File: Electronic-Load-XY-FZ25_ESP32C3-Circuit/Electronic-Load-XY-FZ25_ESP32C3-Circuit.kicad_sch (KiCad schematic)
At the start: 15 parts, among them IC1 BD5334G-TR, J1 Banana-Socket, J2 Banana-Socket, J3 Banana-Socket, J4 Banana-Socket, J5 Conn_1x2_PH, J6 Conn_1x4_PH, J7 Conn_1x2_PH, J8 Conn_1x3_PH, J9 Conn_1x2_PH, Q1 AO3415, U2 Adafruit INA228, U3 SEEEDUINO-XIAO-ESP32C3

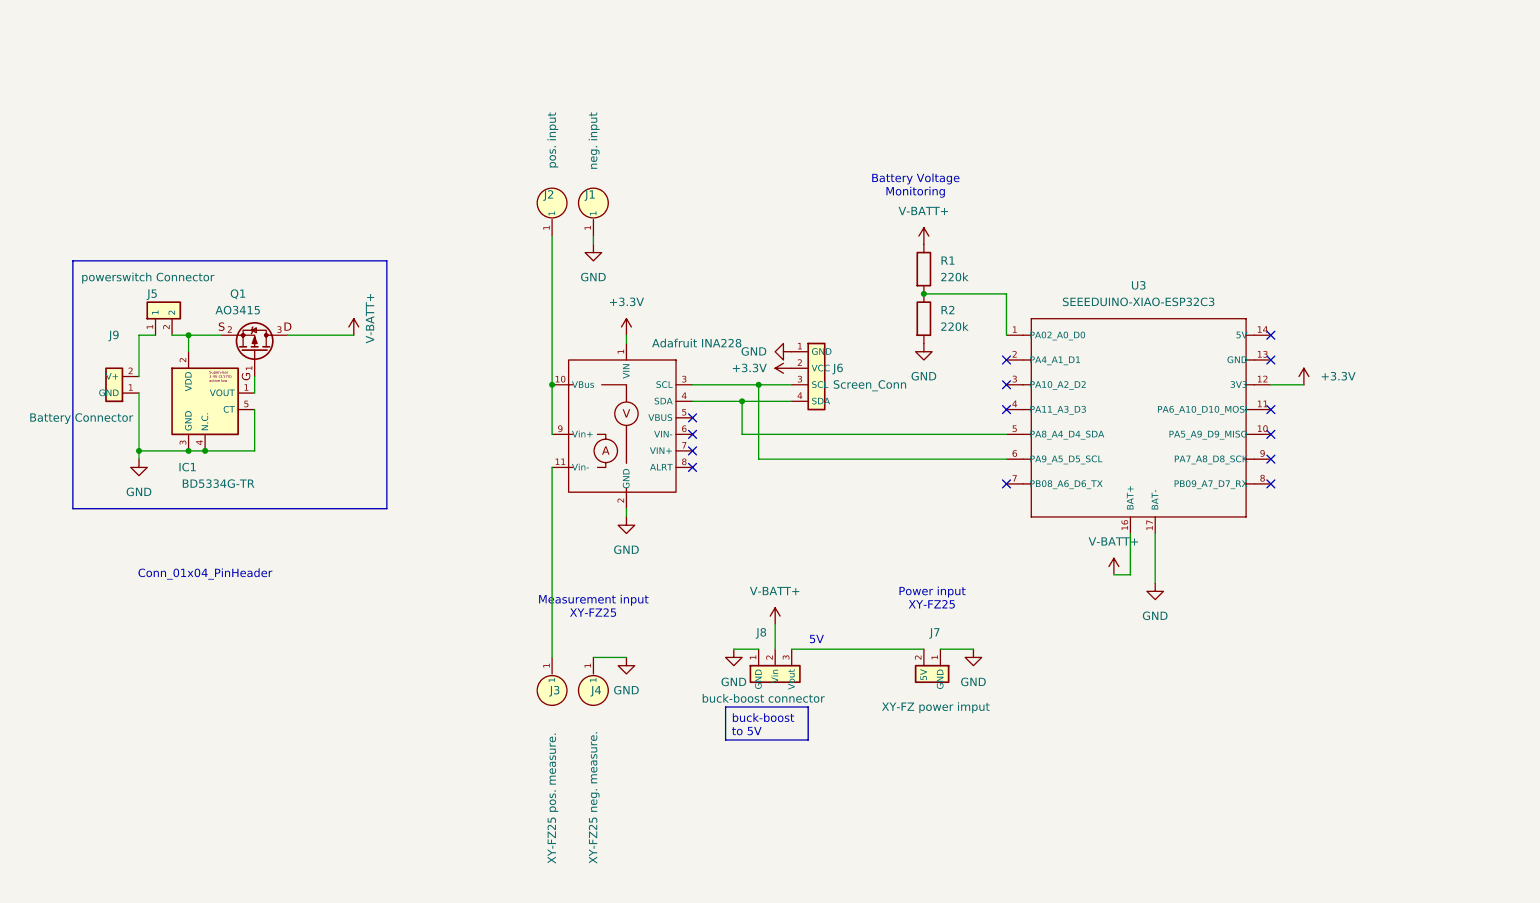
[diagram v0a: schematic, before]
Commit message: Add faulty first design
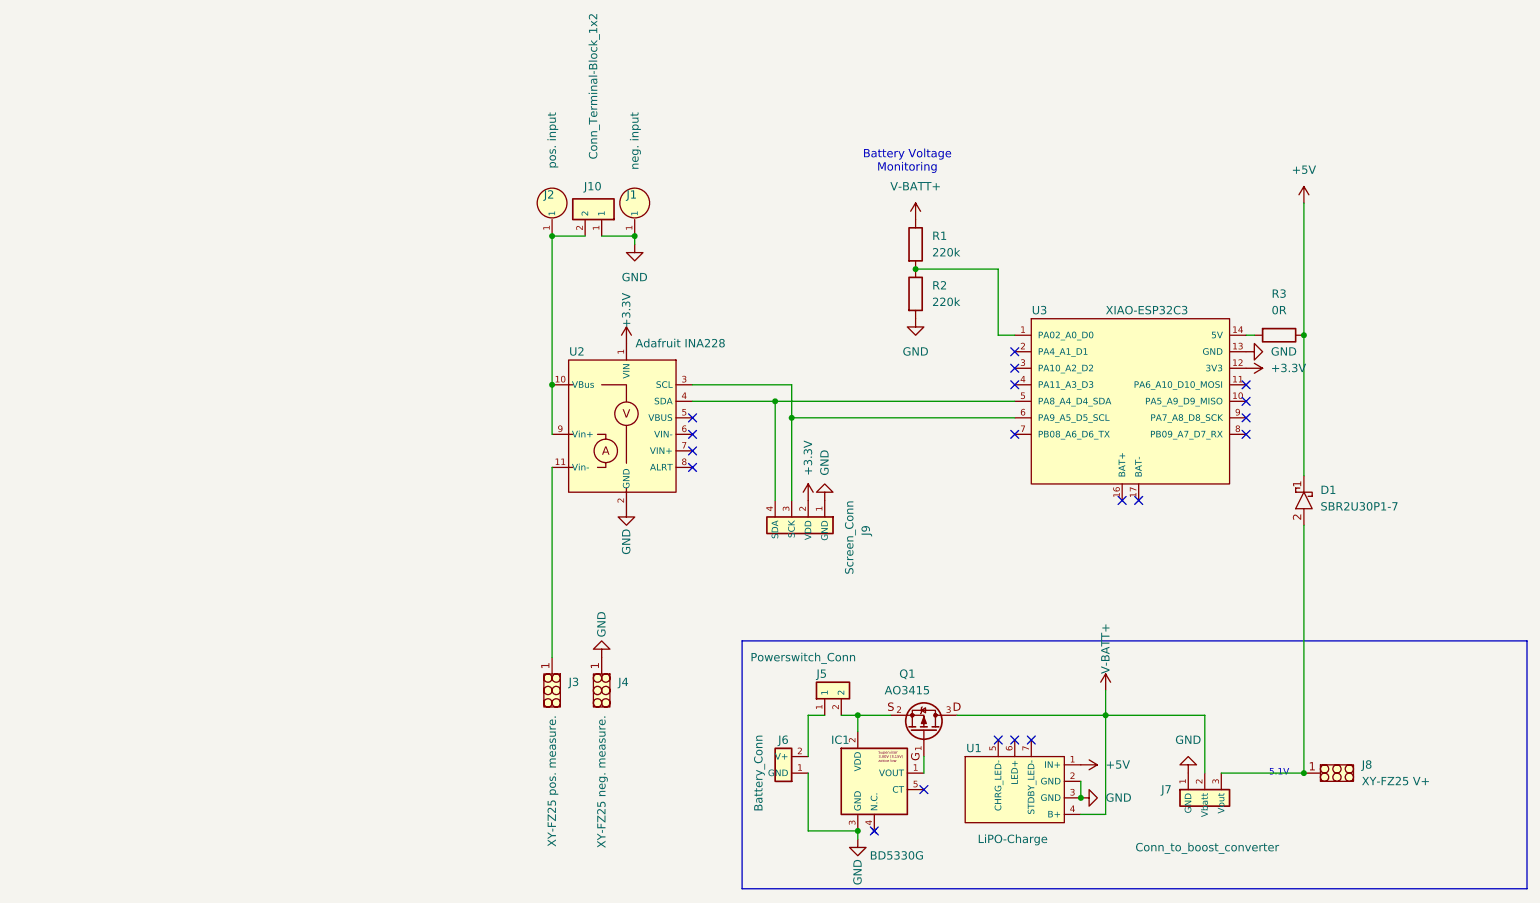
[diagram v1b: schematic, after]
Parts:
- removed IC1: BD5334G-TR, Marcus-PCB-Library:SOT95P280X125-5N, symbol Marcus-PCB-Library:BD5334G-TR
- removed J3, J4: Banana-Socket, Marcus-PCB-Library:banana-socket, symbol Marcus-PCB-Library:Banana-Socket
- removed J7: Conn_1x2_PH, Marcus-PCB-Library:Conn_1x2_PH, symbol Marcus-PCB-Library:Conn_1x2_PH
- removed J8: Conn_1x3_PH, Marcus-PCB-Library:Conn_1x3_PH, symbol Marcus-PCB-Library:Conn_1x3_PH
- added D1: SBR2U30P1-7, Marcus-PCB-Library:SODFL3718X100N, symbol Marcus-PCB-Library:SBR2U30P1-7
- added IC1: BD5330G, SOT95P280X125-5M, symbol Marcus-PCB-Library:BD5330G-2MTR
- added J10: Conn_Terminal-Block_1x2, Marcus-PCB-Library:Conn_Terminal-Block_1x2, symbol Marcus-PCB-Library:Conn_Terminal-Block_1x2
- added J3, J4: mech.-solder-pad_large, Marcus-PCB-Library:Mechc.-solder-pad-large, symbol Marcus-PCB-Library:mechc-solder-pad_large
- added J7: Conn_1x3_PH, Marcus-PCB-Library:Mechc.-solder-pad_1x3, symbol Marcus-PCB-Library:Conn_1x3_PH
- added J8: mech.-solder-pad, Marcus-PCB-Library:Mechc.-solder-pad, symbol Marcus-PCB-Library:mech-solder-pad
- added R3: 0R, Resistor_SMD:R_1206_3216Metric, symbol Device:R
- added U1: LiPO-Charge, Marcus-PCB-Library:TP5000-Charge-IC, symbol Marcus-PCB-Library:TP5000-LiFePO4-Charger
- J5: footprint Marcus-PCB-Library:Conn_1x2_PH -> Marcus-PCB-Library:Mechc.-solder-pad_1x2; SchematicName powerswitch Connector -> Powerswitch_Conn
- J6: renamed from J9; footprint Marcus-PCB-Library:Conn_1x2_PH -> Marcus-PCB-Library:Mechc.-solder-pad_1x2; SchematicName Battery Connector -> Battery_Conn
- U3: value SEEEDUINO-XIAO-ESP32C3 -> XIAO-ESP32C3
- renumbered J6 to J9
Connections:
- net GND: now also U3.13 (GND), IC1.3 (GND), J10.1, J4.1, J7.1 (GND), U1.2 (GND), U1.3 (GND); no longer U3.17 (BAT-)
- net V-BATT+: now also J7.2 (Vbatt), U1.4 (B+); no longer U3.16 (BAT+)
- net at J5.2, Q1.2 (S): now also IC1.2 (VDD)
- net at U3.14 (5V): now also R3.2
- net at J2.1, U2.10 (VBus), U2.9 (Vin+): now also J10.2
- net at U2.11 (Vin-): now also J3.1
- net at Q1.1 (G): now also IC1.1 (VOUT)
- new net: D1.2 (A), J7.3 (Vout), J8.1
- new net +5V: D1.1 (K), R3.1, U1.1 (IN+)
- no-connect marks 14 -> 19
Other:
- note added: "5.1V"
- note removed: "5V"
- note removed: "Conn_01x04_PinHeader"
- note removed: "Measurement input XY-FZ25"
- note removed: "Power input XY-FZ25"
- moved on the sheet: J1, J5, J6, J9, Q1, R1, R2
